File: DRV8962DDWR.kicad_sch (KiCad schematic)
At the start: 10 parts, among them U1 DRV8962DDWR

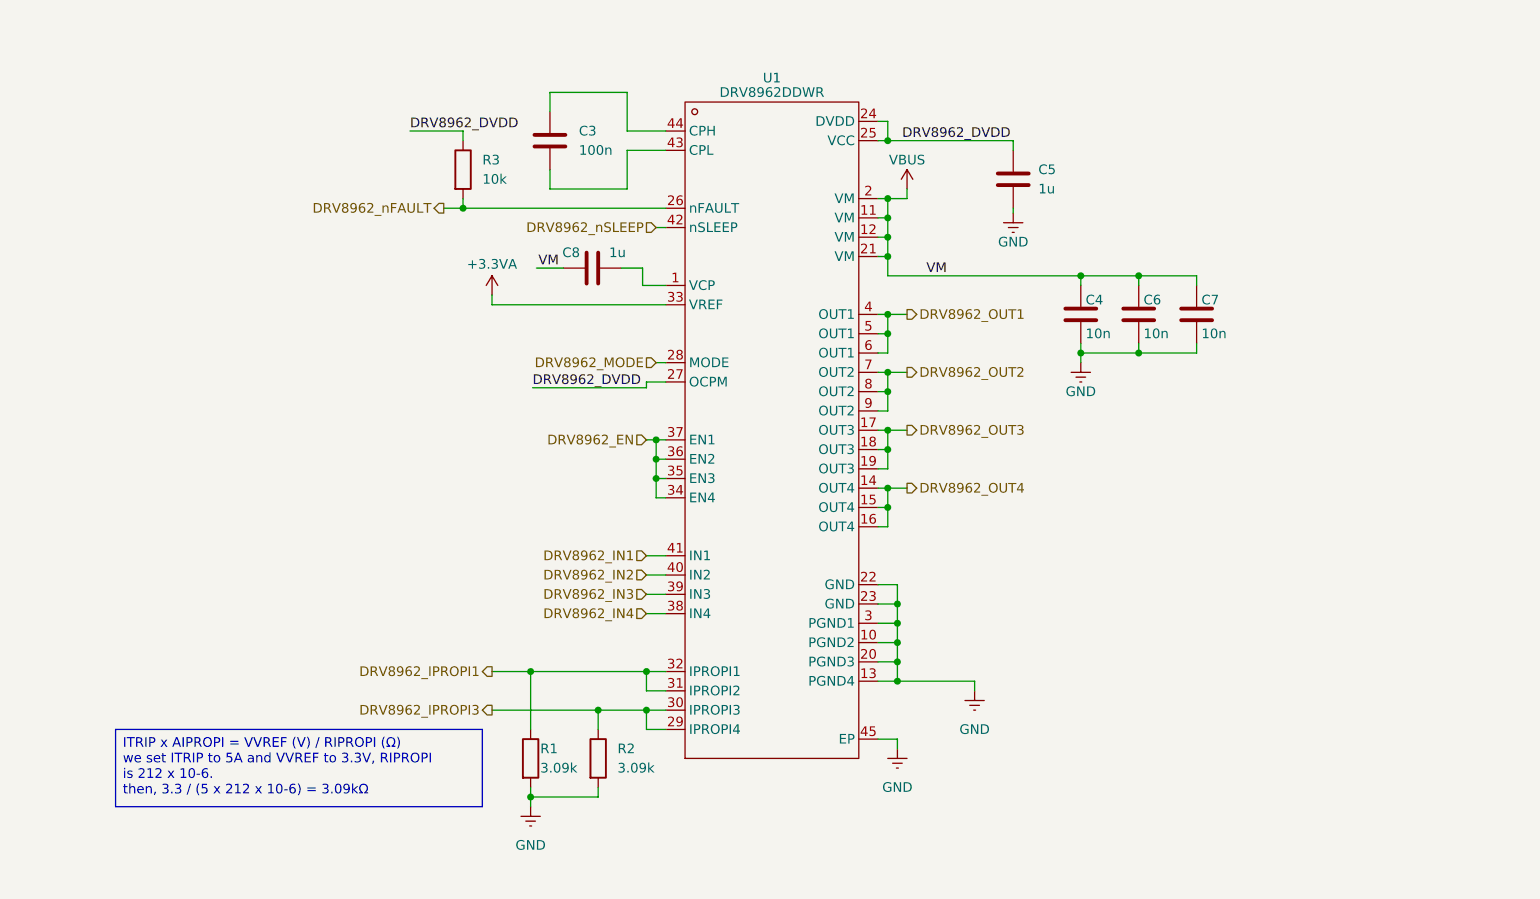
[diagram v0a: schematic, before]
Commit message: change components
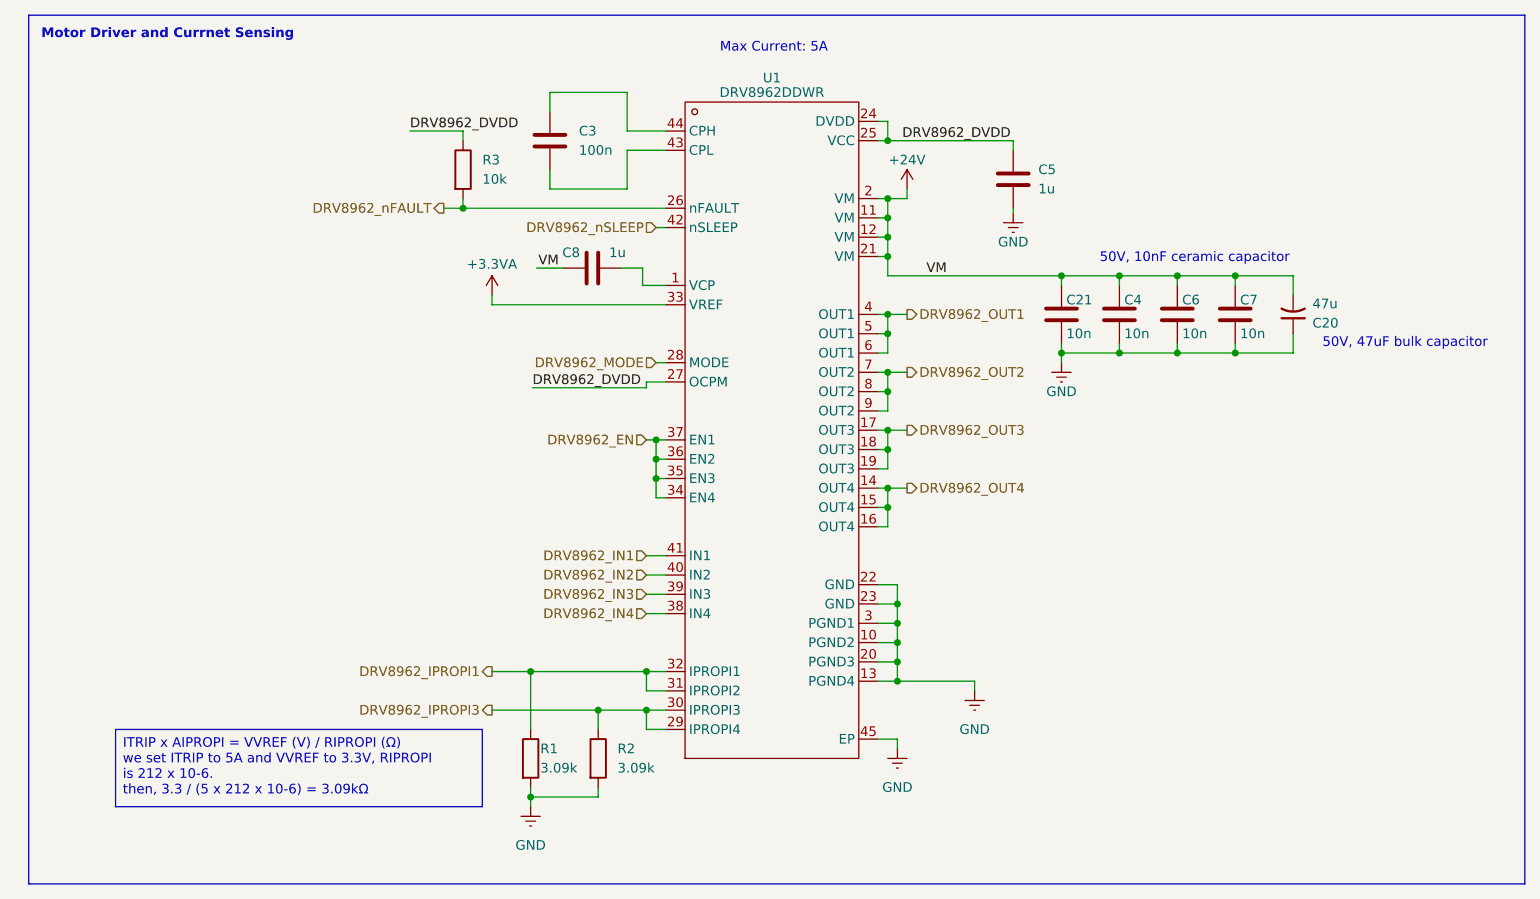
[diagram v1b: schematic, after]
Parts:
- added C20: 47u, Capacitor_SMD:C_0402_1005Metric, symbol Device:C_Small_US
- added C21: 10n, Capacitor_SMD:C_0402_1005Metric, symbol Device:C
- C3, C4, C5, C6, C7, C8: footprint (none) -> Capacitor_SMD:C_0402_1005Metric
- R1, R2, R3: footprint (none) -> PCM_Resistor_SMD_AKL:R_0402_1005Metric
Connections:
- net GND: now also C20.1, C21.2
- net VBUS renamed +24V
- net +24V: now also C20.2, C21.1
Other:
- note added: "50V, 10nF ceramic capacitor"
- note added: "50V, 47uF bulk capacitor"
- note added: "Max Current: 5A"
- note added: "Motor Driver and Currnet Sensing"
- moved on the sheet: C4, C6, C7
